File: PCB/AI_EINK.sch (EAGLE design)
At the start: 172 parts, among them IC3 WM8960, J1 BM04B-GHS-TBT(LF)(SN)(N), J2 C393939, Q1 SI1308EDL-T1-GE3, Q2 DMG2307L, Q3 NMOS_C7465427, T1 MMUN2133LT1G, U1 TPS61092RSAR, U10 AP2112-3.3K, U11 AP2112-3.3K, U12 C233266, U13 TPD4EUSB30DQARDQA10, U14 OPA344, U2 MC74VHC1G14DFT1G, U3 BQ27441DRZR-G1A, U4 BQ24075, U5 MC74VHC1G14DFT1G OR C66196, U6 W25Q128JVSIQSOIC_128JVSIQ_WIN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, U8 MC74VHC1G14DFT1G, U9 EMC2301-1-ACZL-TRMSOP8_MC_MCH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, Y1 ABM8-272-T3

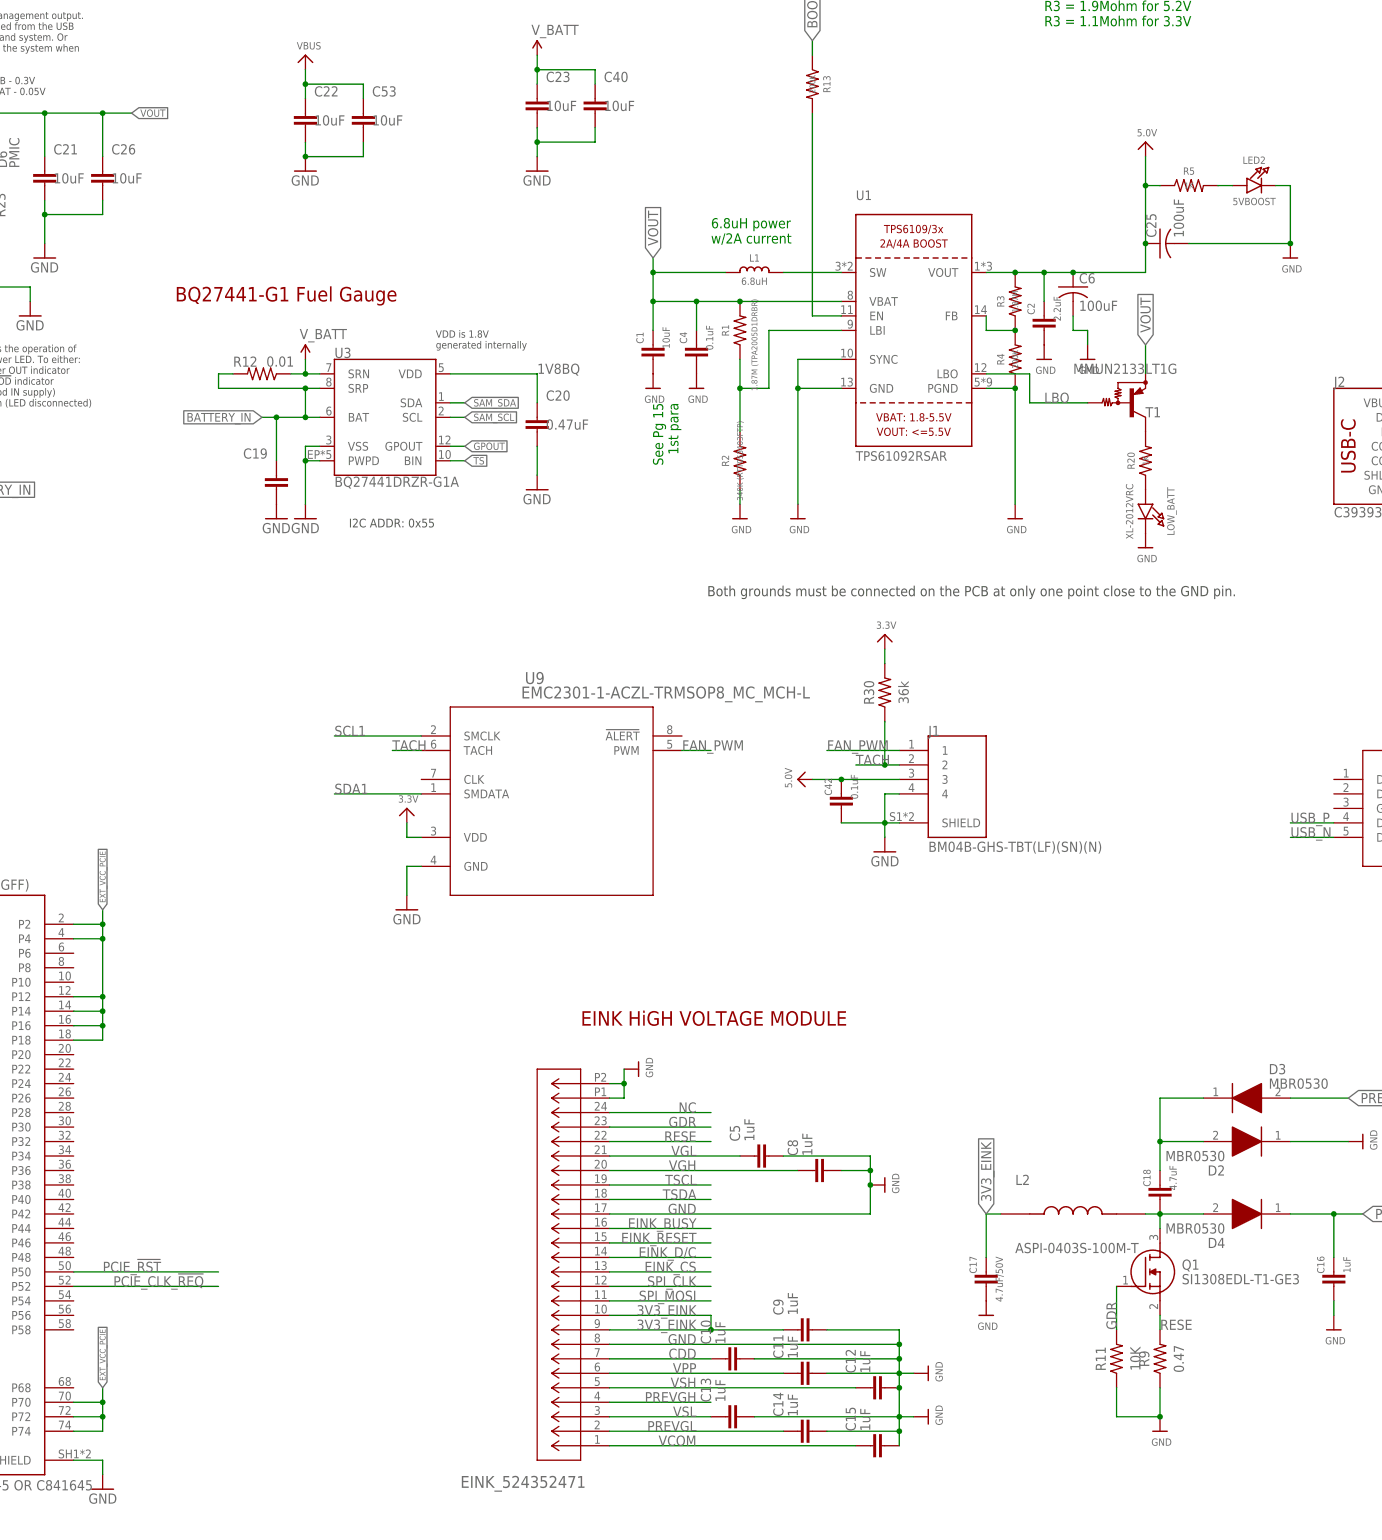
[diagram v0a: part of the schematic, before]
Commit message: pcb
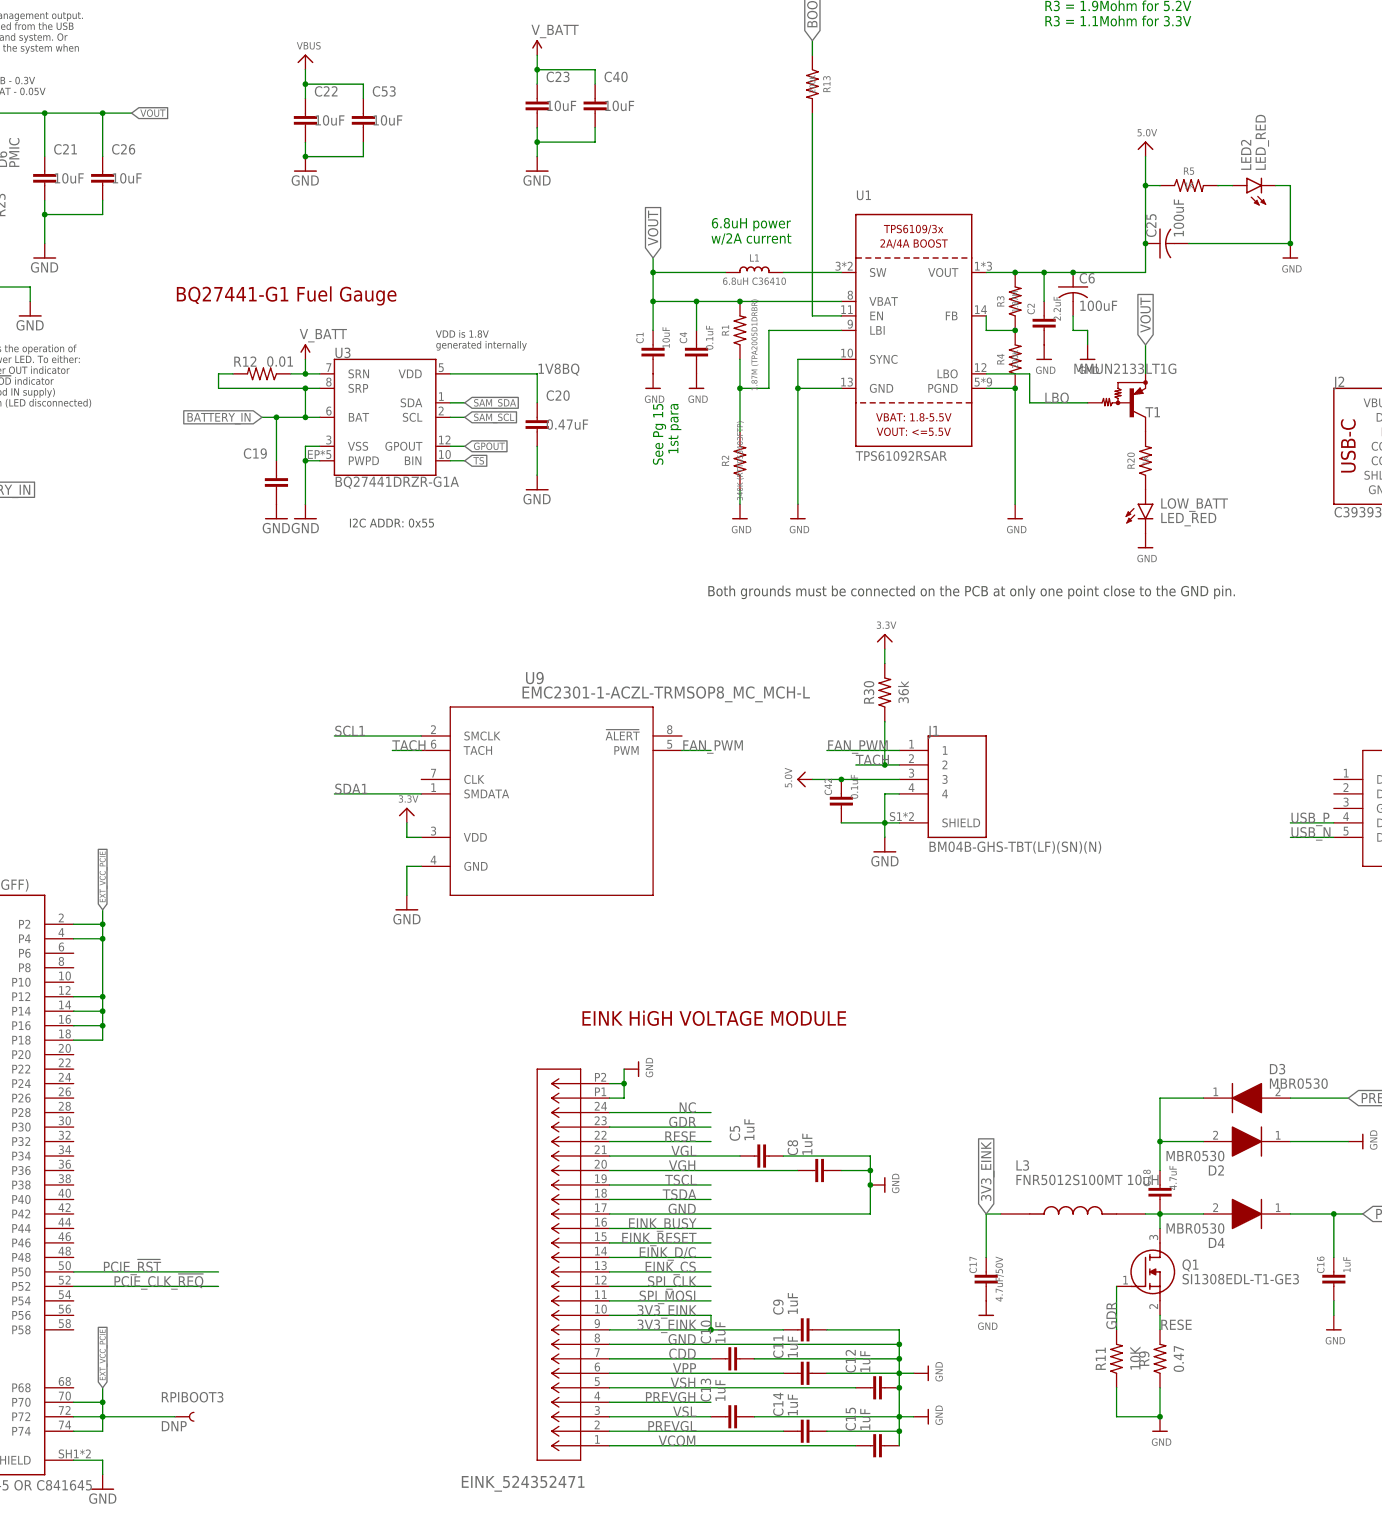
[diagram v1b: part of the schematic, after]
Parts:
- removed L2: ASPI-0403S-100M-T, ASPI-0403S-100M-T:ASPI-0403S-100M-T
- added L3: FNR5012S100MT 10uH, LQH5BPN2R2NT0L:LQH5BPN2R2NT0L
- added RPIBOOT3: DNP, SparkFun-Connectors:TEST-POINT3
- CAMERA: value 524372271CON_524372271_MOL -> C262642
- L1: value 6.8uH -> 6.8uH C36410
- LED2: value 5VBOOST -> LED_RED; device microbuilder:LED0805_NOOUTLINE -> LED:CHIP-ROUND-R_0603
- LOW_BATT: value XL-2012VRC -> LED_RED; device microbuilder:LED0805_NOOUTLINE -> LED:CHIP-ROUND-R_0603
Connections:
- net 3V3_EINK: now also L3.1; no longer L2.1
- net EXT_VCC_PCIE: now also RPIBOOT3.1
- net N$23: now also L3.2; no longer L2.2
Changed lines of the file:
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@@
 <part name="RPI-CM1" library="RPI-CM4" deviceset="RPI-CM4" device="" value="DF40C-100DS-0.4V(51)"/>
 <part name="U1" library="microbuilder" deviceset="VREG_TPS6103X" device="" value="TPS61092RSAR"/>
-<part name="L1" library="microbuilder" deviceset="INDUCTOR" device="TDK_VLC5045" value="6.8uH"/>
+<part name="L1" library="microbuilder" deviceset="INDUCTOR" device="TDK_VLC5045" value="6.8uH C36410"/>
 <part name="U$1" library="microbuilder" deviceset="GND" device=""/>
 <part name="U$2" library="microbuilder" deviceset="GND" device=""/>
@@
 <part name="C2" library="Capacitor" library_urn="urn:adsk.eagle:library:16290819" deviceset="C" device="CHIP-0402(1005-METRIC)" package3d_urn="urn:adsk.eagle:package:16290895/5" technology="_" value="2.2uF"/>
 <part name="U$7" library="microbuilder" deviceset="5.0V" device=""/>
-<part name="LOW_BATT" library="microbuilder" deviceset="LED" device="0805_NOOUTLINE" value="XL-2012VRC"/>
+<part name="LOW_BATT" library="LED" library_urn="urn:adsk.eagle:library:22900745" deviceset="CHIP-ROUND-R" device="_0603" package3d_urn="urn:adsk.eagle:package:24294800/1" value="LED_RED"/>
 <part name="R20" library="Resistor" library_urn="urn:adsk.eagle:library:16378527" deviceset="R-US" device="CHIP-0402(1005-METRIC)" package3d_urn="urn:adsk.eagle:package:16378568/5" technology="_" value="1K"/>
-<part name="LED2" library="microbuilder" deviceset="LED" device="0805_NOOUTLINE" value="5VBOOST"/>
+<part name="LED2" library="LED" library_urn="urn:adsk.eagle:library:22900745" deviceset="CHIP-ROUND-R" device="_0603" package3d_urn="urn:adsk.eagle:package:24294800/1" value="LED_RED"/>
 <part name="R5" library="Resistor" library_urn="urn:adsk.eagle:library:16378527" deviceset="R-US" device="CHIP-0402(1005-METRIC)" package3d_urn="urn:adsk.eagle:package:16378568/5" technology="_" value="1K"/>
 <part name="R13" library="Resistor" library_urn="urn:adsk.eagle:library:16378527" deviceset="R-US" device="CHIP-0402(1005-METRIC)" package3d_urn="urn:adsk.eagle:package:16378568/5" technology="_" value="200K"/>
@@
 <part name="U$83" library="microbuilder" deviceset="GND" device=""/>
 <part name="U$84" library="microbuilder" deviceset="GND" device=""/>
-<part name="L2" library="ASPI-0403S-100M-T" deviceset="ASPI-0403S-100M-T" device=""/>
 <part name="U$85" library="microbuilder" deviceset="GND" device=""/>
 <part name="U$86" library="microbuilder" deviceset="GND" device=""/>
@@
 <part name="GND10" library="supply1" deviceset="GND" device=""/>
 <part name="JOY_STICK" library="BM04B-GHS-TBT_LF__SN__N_" deviceset="BM04B-GHS-TBT(LF)(SN)(N)" device=""/>
-<part name="CAMERA" library="2024-03-29_02-21-27_Library" deviceset="524372271" device="CON_524372271_MOL"/>
+<part name="CAMERA" library="2024-03-29_02-21-27_Library" deviceset="524372271" device="CON_524372271_MOL" value="C262642"/>
 <part name="GND11" library="SparkFun-Aesthetics" deviceset="GND" device=""/>
 <part name="Q2" library="DMG2307L" deviceset="DMG2307L" device="" value="DMG2307L"/>
@@
 <part name="R43" library="Resistor" library_urn="urn:adsk.eagle:library:16378527" deviceset="R-US" device="CHIP-0402(1005-METRIC)" package3d_urn="urn:adsk.eagle:package:16378568/5" technology="_" value="10K"/>
 <part name="R44" library="Resistor" library_urn="urn:adsk.eagle:library:16378527" deviceset="R-US" device="CHIP-0402(1005-METRIC)" package3d_urn="urn:adsk.eagle:package:16378568/5" technology="_" value="6.57k"/>
+<part name="RPIBOOT3" library="SparkFun-Connectors" deviceset="TEST-POINT" device="3" value="DNP"/>
+<part name="L3" library="LQH5BPN2R2NT0L" deviceset="LQH5BPN2R2NT0L" device="" value="FNR5012S100MT 10uH"/>
 </parts>
 <sheets>
@@
 <attribute name="VALUE" x="590.296" y="260.096" size="1.27" layer="96"/>
 </instance>
-<instance part="LOW_BATT" gate="G$1" x="591.82" y="193.04" smashed="yes" rot="R270">
-<attribute name="NAME" x="596.265" y="194.31" size="1.27" layer="95" rot="R270" align="center"/>
-<attribute name="VALUE" x="589.026" y="194.31" size="1.27" layer="96" rot="R270" align="center"/>
+<instance part="LOW_BATT" gate="G$1" x="591.82" y="195.58" smashed="yes">
+<attribute name="NAME" x="594.36" y="194.818" size="1.778" layer="95" rot="R180" align="top-right"/>
+<attribute name="VALUE" x="594.36" y="192.278" size="1.778" layer="96" rot="R180" align="top-right"/>
 </instance>
 <instance part="R20" gate="G$1" x="591.82" y="203.2" smashed="yes" rot="R90">
@@
 <attribute name="VALUE" x="591.82" y="203.2" size="1.016" layer="96" font="vector" ratio="15" rot="R90" align="center"/>
 </instance>
-<instance part="LED2" gate="G$1" x="612.14" y="251.46" smashed="yes">
-<attribute name="NAME" x="610.87" y="255.905" size="1.27" layer="95" align="center"/>
-<attribute name="VALUE" x="610.87" y="248.666" size="1.27" layer="96" align="center"/>
+<instance part="LED2" gate="G$1" x="609.6" y="251.46" smashed="yes" rot="R90">
+<attribute name="NAME" x="610.362" y="254" size="1.778" layer="95" rot="R270" align="top-right"/>
+<attribute name="VALUE" x="612.902" y="254" size="1.778" layer="96" rot="R270" align="top-right"/>
 </instance>
 <instance part="R5" gate="G$1" x="599.44" y="251.46" smashed="yes">
@@
 <attribute name="VALUE" x="623.316" y="48.26" size="1.27" layer="96"/>
 </instance>
-<instance part="L2" gate="G$1" x="579.12" y="71.12" smashed="yes">
-<attribute name="NAME" x="568.96" y="76.2" size="1.778" layer="95"/>
-<attribute name="VALUE" x="568.96" y="66.04" size="1.778" layer="96" align="top-left"/>
-</instance>
 <instance part="U$85" gate="G$1" x="594.36" y="33.02" smashed="yes">
 <attribute name="VALUE" x="592.836" y="30.48" size="1.27" layer="96"/>
@@
 <attribute name="VALUE" x="551.18" y="-4.318" size="1.778" layer="96" rot="R180" align="center"/>
 </instance>
+<instance part="RPIBOOT3" gate="G$1" x="421.64" y="35.56" smashed="yes">
+<attribute name="NAME" x="419.1" y="38.1" size="1.778" layer="95" font="vector"/>
+<attribute name="VALUE" x="419.1" y="33.02" size="1.778" layer="96" font="vector"/>
+</instance>
+<instance part="L3" gate="G$1" x="579.12" y="71.12" smashed="yes">
+<attribute name="NAME" x="568.96" y="78.74" size="1.778" layer="95"/>
+<attribute name="VALUE" x="568.96" y="76.2" size="1.778" layer="96"/>
+</instance>
 </instances>
 <busses>
@@
 <wire x1="601.98" y1="71.12" x2="594.36" y2="71.12" width="0.1524" layer="91"/>
 <junction x="594.36" y="71.12"/>
-<pinref part="L2" gate="G$1" pin="2"/>
 <wire x1="594.36" y1="71.12" x2="591.82" y2="71.12" width="0.1524" layer="91"/>
+<pinref part="L3" gate="G$1" pin="2"/>
 </segment>
 </net>
@@
 </segment>
 <segment>
-<pinref part="L2" gate="G$1" pin="1"/>
 <wire x1="566.42" y1="71.12" x2="563.88" y2="71.12" width="0.1524" layer="91"/>
 <wire x1="563.88" y1="71.12" x2="563.88" y2="63.5" width="0.1524" layer="91"/>
 <pinref part="C17" gate="G$1" pin="1"/>
 <label x="563.88" y="71.12" size="1.778" layer="95" rot="R90" xref="yes"/>
+<pinref part="L3" gate="G$1" pin="1"/>
 </segment>
 </net>
@@
 <junction x="408.94" y="38.1"/>
 <label x="408.94" y="40.64" size="1.016" layer="95" rot="R90" xref="yes"/>
+<pinref part="RPIBOOT3" gate="G$1" pin="1"/>
+<wire x1="421.64" y1="35.56" x2="408.94" y2="35.56" width="0.1524" layer="91"/>
 </segment>
 </net>
